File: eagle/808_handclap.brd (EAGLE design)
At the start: 100 x 80 mm, 82 parts, among them IC1 LM339N, IC2 TL071P, IC3 TL071P, Q1 2N3906, Q2 2N3904, Q3 2N3906, Q4 2N3906, Q5 2N3904, Q6 2N3904, Q7 2N3904, U1 POWER, U22 BA6110SIL

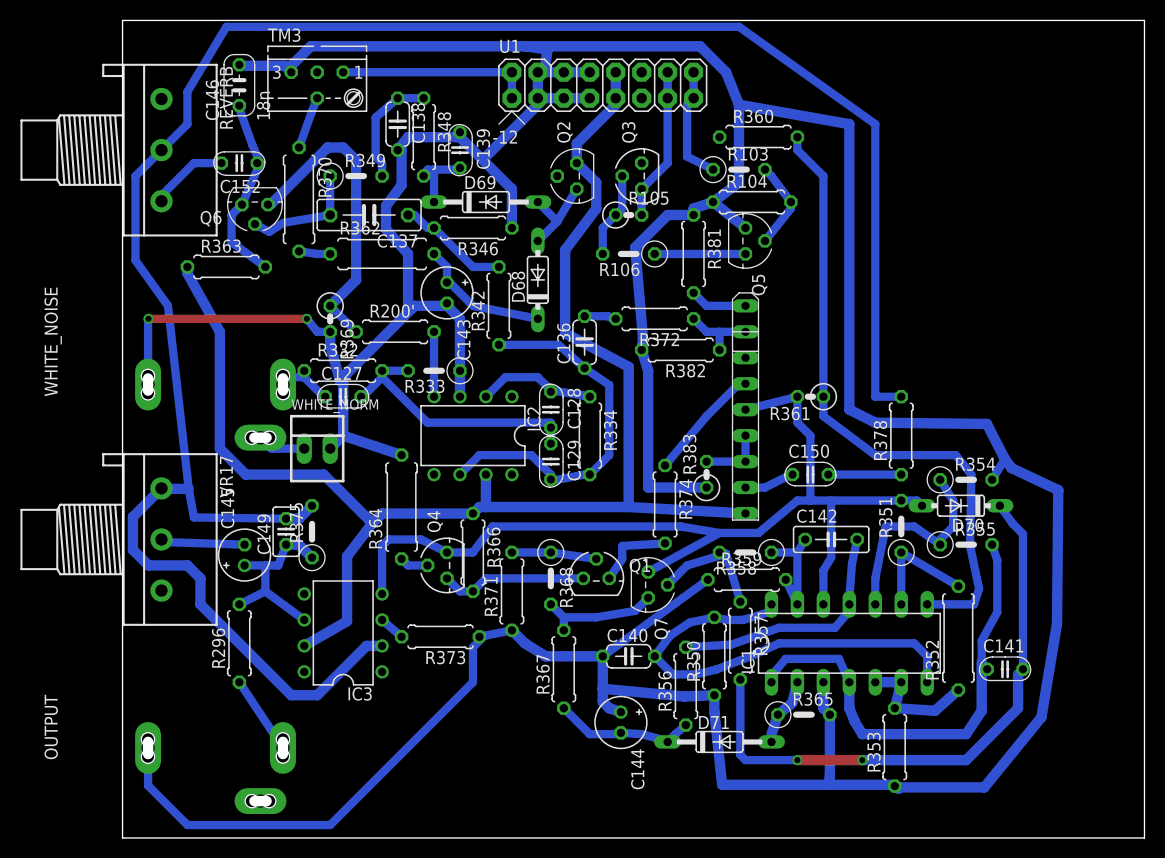
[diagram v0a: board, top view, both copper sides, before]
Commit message: routed
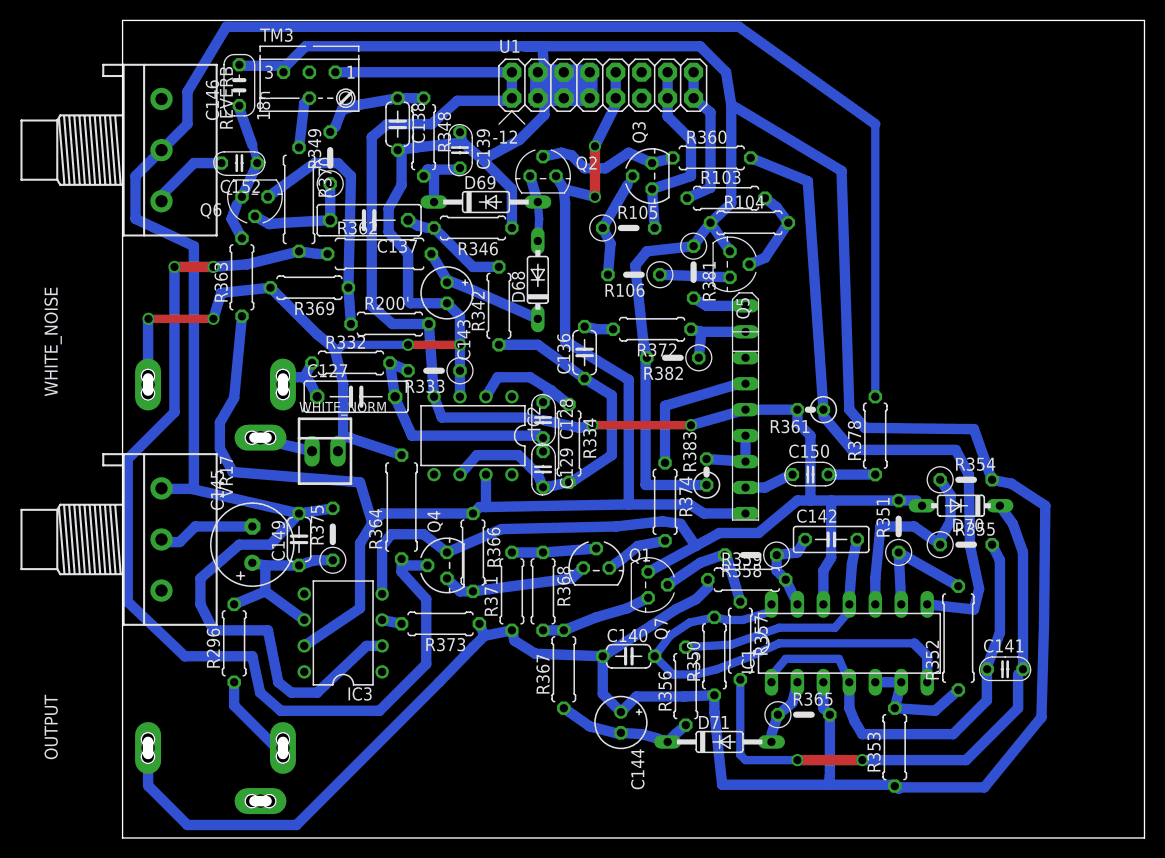
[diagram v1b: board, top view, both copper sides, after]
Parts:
- C127: device TR808clone:C035-025X75 -> TR808clone:C075-032X103
- C145: device TR808clone:E2-5 -> TR808clone:E3,5-8
- C149: device TR808clone:C025-025X050 -> TR808clone:C050-024X044
- R103, R368: device TR808clone:0207/5V -> TR808clone:0207/7
- R105: device TR808clone:0207/2V -> TR808clone:0207/5V
- R369: device TR808clone:0207/2V -> TR808clone:0207/7
- R381, R382: device TR808clone:0207/7 -> TR808clone:0207/5V
- moved R360 5.00 mm to (57.7, 66.5)
- moved R369 3.66 mm to (18.3, 53.8), turned to 180 degrees
- moved Q2 3.30 mm to (41.1, 64.8), turned to 0 degrees
- moved R349 3.10 mm to (20.3, 66.5), turned to 90 degrees
- moved R103 3.07 mm to (59.1, 62.6)
- moved Q5 2.75 mm to (59.4, 56.1)
- moved R378 2.54 mm to (73.7, 39.4)
- moved R334 2.17 mm to (43.7, 38.6)
- moved R106 2.09 mm to (50.0, 55.1)
- moved R375 2.05 mm to (20.6, 29.7)
- moved R104 2.05 mm to (61.3, 60.2)
- moved R363 1.83 mm to (11.7, 54.9), turned to 90 degrees
- moved R381 1.78 mm to (55.9, 55.4)
- moved C149 1.48 mm to (17.3, 29.2)
- moved R368 1.48 mm to (41.1, 24.1)
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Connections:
- net N$52: now also C127.2; no longer C127.P$2
- net WN: now also C127.1; no longer C127.P$1
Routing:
- net N$48: track 5.87 -> 100.6 mm, vias 0 -> 2
- net -12V: track 121.1 -> 189.9 mm, vias 0 -> 2
- net N$43: track 0.00 -> 14.0 mm
- net GND: track 468.1 -> 461.9 mm, vias 2 -> 4
- net N$42: track 30.3 -> 24.2 mm
- net N$46: track 18.9 -> 14.1 mm
- net TRIG: track 15.0 -> 18.9 mm
- net CP: track 11.4 -> 14.6 mm
- net N$78: track 11.8 -> 8.98 mm
- net N$44: track 9.09 -> 6.47 mm
- net N$62: track 7.14 -> 4.60 mm
- net N$52: track 26.4 -> 24.0 mm
- net N$60: track 11.4 -> 13.8 mm
- net N$37: track 8.41 -> 10.6 mm
- net N$3: track 8.89 -> 6.86 mm
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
